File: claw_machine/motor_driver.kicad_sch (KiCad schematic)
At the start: 3 parts, among them J701 Screw_Terminal_01x02, J702 Screw_Terminal_01x02, U701 L298N

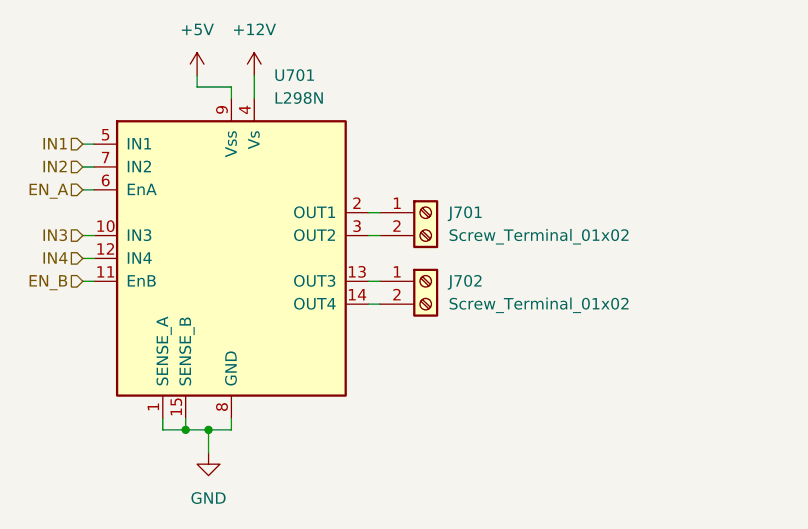
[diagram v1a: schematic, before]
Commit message: Finish, Gerbers
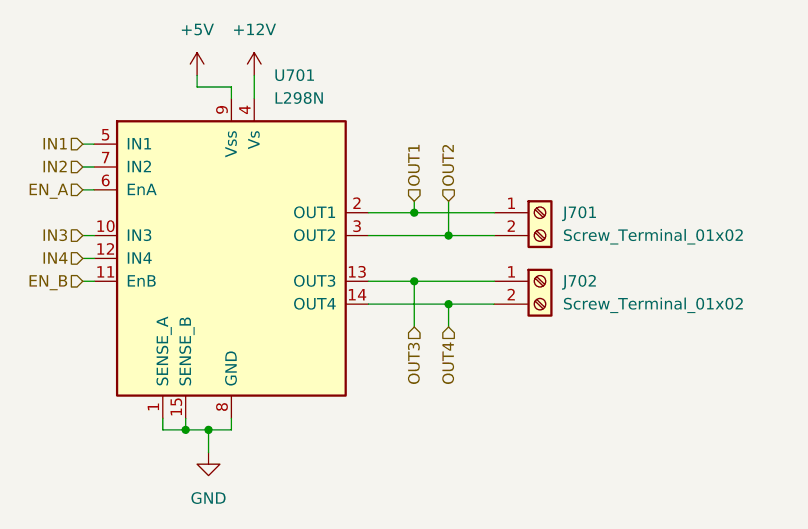
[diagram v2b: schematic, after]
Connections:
- net  OUT3: now reaches J702.1 (Pin_1), U701.13 (OUT3)
- net  OUT4: now reaches J702.2 (Pin_2), U701.14 (OUT4)
- net  OUT1: now reaches J701.1 (Pin_1), U701.2 (OUT1)
- net  OUT2: now reaches J701.2 (Pin_2), U701.3 (OUT2)
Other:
- moved on the sheet: J701, J702
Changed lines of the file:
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@@
   (junction (at 74.93 76.2) (diameter 0) (color 0 0 0 0)
   )
+  (junction (at 97.79 52.07) (diameter 0) (color 0 0 0 0)
+  )
+  (junction (at 97.79 59.69) (diameter 0) (color 0 0 0 0)
+  )
+  (junction (at 101.6 62.23) (diameter 0) (color 0 0 0 0)
+  )
   (junction (at 72.39 76.2) (diameter 0) (color 0 0 0 0)
   )
-  (wire (pts (xy 92.71 52.07) (xy 93.98 52.07))
+  (junction (at 101.6 54.61) (diameter 0) (color 0 0 0 0)
+  )
+  (wire (pts (xy 101.6 50.8) (xy 101.6 54.61))
+    (stroke (width 0) (type default))
+  )
+  (wire (pts (xy 97.79 52.07) (xy 106.68 52.07))
+    (stroke (width 0) (type default))
+  )
+  (wire (pts (xy 97.79 50.8) (xy 97.79 52.07))
+    (stroke (width 0) (type default))
+  )
+  (wire (pts (xy 92.71 52.07) (xy 97.79 52.07))
     (stroke (width 0) (type default))
   )
@@
     (stroke (width 0) (type default))
   )
+  (wire (pts (xy 101.6 62.23) (xy 101.6 64.77))
+    (stroke (width 0) (type default))
+  )
+  (wire (pts (xy 101.6 62.23) (xy 106.68 62.23))
+    (stroke (width 0) (type default))
+  )
   (wire (pts (xy 60.96 44.45) (xy 62.23 44.45))
     (stroke (width 0) (type default))
   )
+  (wire (pts (xy 97.79 59.69) (xy 106.68 59.69))
+    (stroke (width 0) (type default))
+  )
+  (wire (pts (xy 97.79 59.69) (xy 97.79 64.77))
+    (stroke (width 0) (type default))
+  )
   (wire (pts (xy 80.01 36.83) (xy 80.01 39.37))
     (stroke (width 0) (type default))
@@
     (stroke (width 0) (type default))
   )
-  (wire (pts (xy 92.71 59.69) (xy 93.98 59.69))
+  (wire (pts (xy 101.6 54.61) (xy 106.68 54.61))
+    (stroke (width 0) (type default))
+  )
+  (wire (pts (xy 92.71 59.69) (xy 97.79 59.69))
     (stroke (width 0) (type default))
   )
@@
     (stroke (width 0) (type default))
   )
-  (wire (pts (xy 92.71 62.23) (xy 93.98 62.23))
+  (wire (pts (xy 92.71 62.23) (xy 101.6 62.23))
     (stroke (width 0) (type default))
   )
@@
     (stroke (width 0) (type default))
   )
-  (wire (pts (xy 92.71 54.61) (xy 93.98 54.61))
+  (wire (pts (xy 92.71 54.61) (xy 101.6 54.61))
     (stroke (width 0) (type default))
   )
@@
     (stroke (width 0) (type default))
   )
+  (hierarchical_label " OUT4" (shape input) (at 101.6 64.77 270) (fields_autoplaced)
+    (effects (font (size 1.27 1.27)) (justify right))
+  )
   (hierarchical_label "IN2" (shape input) (at 60.96 46.99 180) (fields_autoplaced)
     (effects (font (size 1.27 1.27)) (justify right))
   )
+  (hierarchical_label " OUT3" (shape input) (at 97.79 64.77 270) (fields_autoplaced)
+    (effects (font (size 1.27 1.27)) (justify right))
+  )
+  (hierarchical_label " OUT1" (shape input) (at 97.79 50.8 90) (fields_autoplaced)
+    (effects (font (size 1.27 1.27)) (justify left))
+  )
   (hierarchical_label "IN3" (shape input) (at 60.96 54.61 180) (fields_autoplaced)
     (effects (font (size 1.27 1.27)) (justify right))
@@
   (hierarchical_label "IN1" (shape input) (at 60.96 44.45 180) (fields_autoplaced)
     (effects (font (size 1.27 1.27)) (justify right))
+  )
+  (hierarchical_label " OUT2" (shape input) (at 101.6 50.8 90) (fields_autoplaced)
+    (effects (font (size 1.27 1.27)) (justify left))
   )
   (hierarchical_label "IN4" (shape input) (at 60.96 57.15 180) (fields_autoplaced)
@@
           (reference "U701") (unit 1)
         )
-        (path "/2e48e9a4-e55f-4bd7-8086-6a8b9c5eabc1/a5b51e80-e745-4cc8-8f69-0457f2fb6018"
-          (reference "U601") (unit 1)
-        )
       )
       (project "ClawMachine"
@@
           (reference "#PWR0702") (unit 1)
         )
-        (path "/2e48e9a4-e55f-4bd7-8086-6a8b9c5eabc1/a5b51e80-e745-4cc8-8f69-0457f2fb6018"
-          (reference "#PWR0602") (unit 1)
-        )
       )
       (project "ClawMachine"
@@
     )
   )
-  (symbol (lib_id "Connector:Screw_Terminal_01x02") (at 99.06 52.07 0) (unit 1)
-    (in_bom yes) (on_board yes) (dnp no) (fields_autoplaced)
-    (property "Reference" "J701" (at 101.6 52.07 0)
-      (effects (font (size 1.27 1.27)) (justify left))
-    )
-    (property "Value" "Screw_Terminal_01x02" (at 101.6 54.61 0)
-      (effects (font (size 1.27 1.27)) (justify left))
-    )
-    (property "Footprint" "TerminalBlock:TerminalBlock_bornier-2_P5.08mm" (at 99.06 52.07 0)
-      (effects (font (size 1.27 1.27)) hide)
-    )
-    (property "Datasheet" "~" (at 99.06 52.07 0)
+  (symbol (lib_id "Connector:Screw_Terminal_01x02") (at 111.76 52.07 0) (unit 1)
+    (in_bom yes) (on_board yes) (dnp no) (fields_autoplaced)
+    (property "Reference" "J701" (at 114.3 52.07 0)
+      (effects (font (size 1.27 1.27)) (justify left))
+    )
+    (property "Value" "Screw_Terminal_01x02" (at 114.3 54.61 0)
+      (effects (font (size 1.27 1.27)) (justify left))
+    )
+    (property "Footprint" "TerminalBlock:TerminalBlock_bornier-2_P5.08mm" (at 111.76 52.07 0)
+      (effects (font (size 1.27 1.27)) hide)
+    )
+    (property "Datasheet" "~" (at 111.76 52.07 0)
       (effects (font (size 1.27 1.27)) hide)
     )
@@
         (path "/2e48e9a4-e55f-4bd7-8086-6a8b9c5eabc1/bb6e873f-fe99-4b0f-a00a-430ca8ec6fa2"
           (reference "J701") (unit 1)
-        )
-        (path "/2e48e9a4-e55f-4bd7-8086-6a8b9c5eabc1/a5b51e80-e745-4cc8-8f69-0457f2fb6018"
-          (reference "J601") (unit 1)
         )
       )
@@
           (reference "#PWR0703") (unit 1)
         )
-        (path "/2e48e9a4-e55f-4bd7-8086-6a8b9c5eabc1/a5b51e80-e745-4cc8-8f69-0457f2fb6018"
-          (reference "#PWR0603") (unit 1)
-        )
       )
       (project "ClawMachine"
@@
           (reference "#PWR0701") (unit 1)
         )
-        (path "/2e48e9a4-e55f-4bd7-8086-6a8b9c5eabc1/a5b51e80-e745-4cc8-8f69-0457f2fb6018"
-          (reference "#PWR0601") (unit 1)
-        )
       )
       (project "ClawMachine"
@@
     )
   )
-  (symbol (lib_id "Connector:Screw_Terminal_01x02") (at 99.06 59.69 0) (unit 1)
-    (in_bom yes) (on_board yes) (dnp no) (fields_autoplaced)
-    (property "Reference" "J702" (at 101.6 59.69 0)
-      (effects (font (size 1.27 1.27)) (justify left))
-    )
-    (property "Value" "Screw_Terminal_01x02" (at 101.6 62.23 0)
-      (effects (font (size 1.27 1.27)) (justify left))
-    )
-    (property "Footprint" "TerminalBlock:TerminalBlock_bornier-2_P5.08mm" (at 99.06 59.69 0)
-      (effects (font (size 1.27 1.27)) hide)
-    )
-    (property "Datasheet" "~" (at 99.06 59.69 0)
+  (symbol (lib_id "Connector:Screw_Terminal_01x02") (at 111.76 59.69 0) (unit 1)
+    (in_bom yes) (on_board yes) (dnp no) (fields_autoplaced)
+    (property "Reference" "J702" (at 114.3 59.69 0)
+      (effects (font (size 1.27 1.27)) (justify left))
+    )
+    (property "Value" "Screw_Terminal_01x02" (at 114.3 62.23 0)
+      (effects (font (size 1.27 1.27)) (justify left))
+    )
+    (property "Footprint" "TerminalBlock:TerminalBlock_bornier-2_P5.08mm" (at 111.76 59.69 0)
+      (effects (font (size 1.27 1.27)) hide)
+    )
+    (property "Datasheet" "~" (at 111.76 59.69 0)
       (effects (font (size 1.27 1.27)) hide)
     )
@@
           (reference "J702") (unit 1)
         )
-        (path "/2e48e9a4-e55f-4bd7-8086-6a8b9c5eabc1/a5b51e80-e745-4cc8-8f69-0457f2fb6018"
-          (reference "J602") (unit 1)
-        )
-      )
+      )
